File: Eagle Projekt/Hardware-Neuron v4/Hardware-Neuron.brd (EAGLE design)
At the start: 76.2 x 98.7 mm, 118 parts, among them Q1 FDN360P, Q10 BSS123, Q11 BSS123, Q12 BSS123, Q13 FDN360P, Q14 BCX71SMD, Q15 BCX71SMD, Q16 BSS123, Q17 BSS123, Q18 BSS123, Q19 BSS123, Q2 BCX71SMD, Q20 BSS123, Q21 BSS123, Q22 BCX71SMD, Q23 BCX71SMD, Q24 BSS123, Q25 BSS123, Q26 BSS123, Q27 BSS123, Q28 BSS123, Q29 BSS123, Q3 BCX71SMD, Q30 BSS123, Q31 BSS123, Q32 BSS123, Q33 BSS123, Q34 BSS123, Q35 BSS123, Q36 BSS123, Q37 BSS123, Q4 FDN360P, Q5 FDN360P, Q6 BSS123, Q7 BSS123, Q8 BSS123, Q9 FDN360P, T1 BC846, T2 BC846, T3 BC846, T4 BC846, T5 BC846, T6 BC846, T7 BC846, T8 BC846

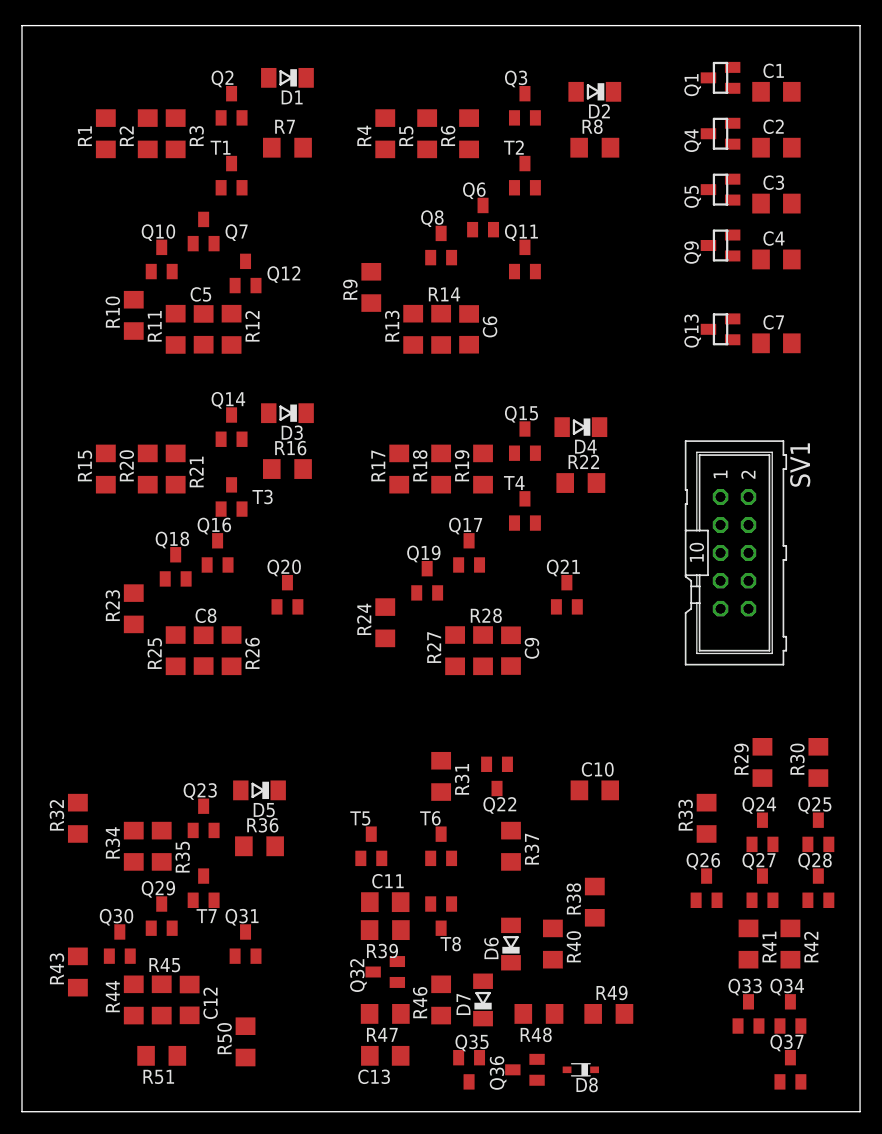
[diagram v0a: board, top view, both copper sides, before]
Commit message: Layout upgrade
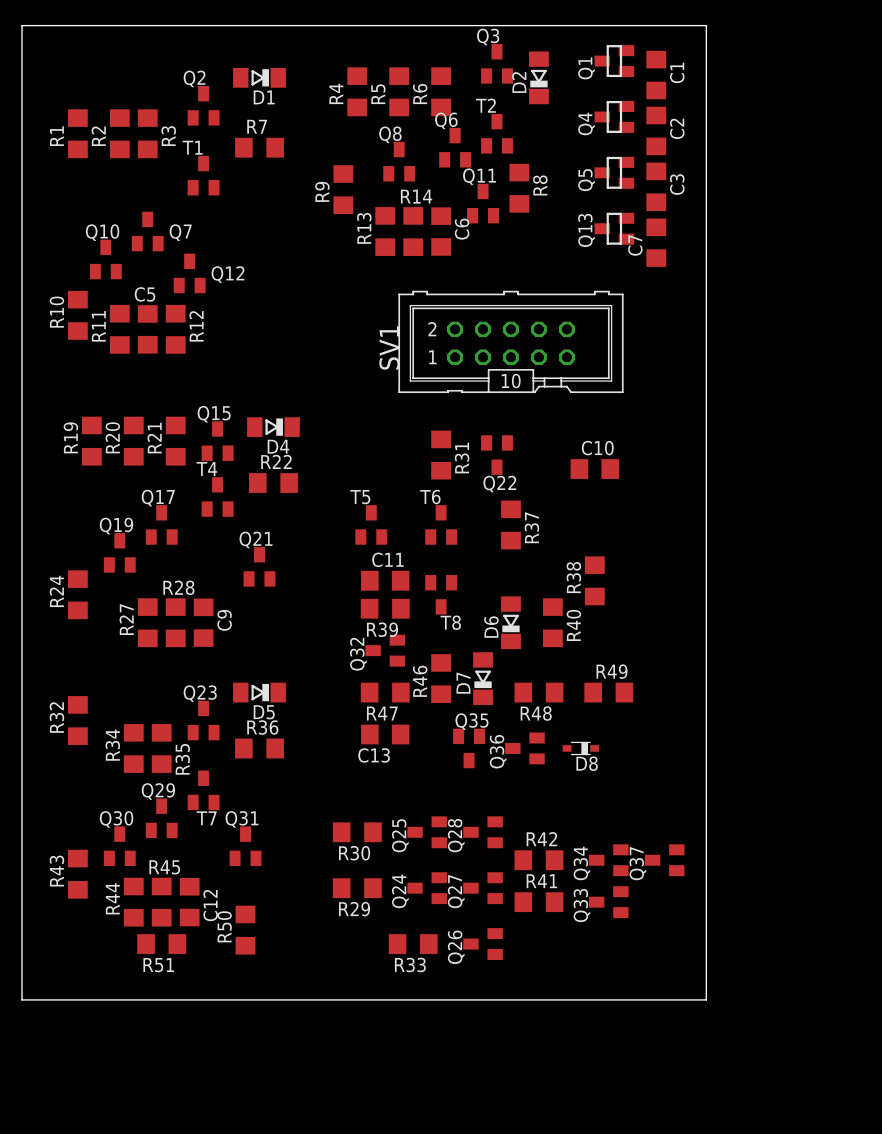
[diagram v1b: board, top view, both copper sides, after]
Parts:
- removed C4: 10n, rcl:C1206
- removed C8: 100n, rcl:C1206
- removed D3: PMLL41SOD80C, diode:SOD80C
- removed Q14: BCX71SMD, transistor-pnp:SOT23
- removed Q16, Q18, Q20: BSS123, transistor-small-signal:SOT23
- removed Q9: FDN360P, transistor-power:SUPER-SOT3
- removed R15, R17, R18, R23, R25, R26: 1kE, rcl:R1206
- removed R16: 10ME, rcl:R1206
- removed T3: BC846, transistor:SOT23
- moved R30 42.4 mm to (30.5, 25.4), turned to 180 degrees
- moved R29 38.6 mm to (30.5, 20.3), turned to 180 degrees
- moved R19 35.7 mm to (6.35, 61.0)
- moved Q25 35.6 mm to (36.8, 25.4), turned to 90 degrees
- moved Q24 30.9 mm to (36.8, 20.3), turned to 90 degrees
- moved Q28 30.9 mm to (41.9, 25.4), turned to 90 degrees
- moved D8 29.2 mm to (50.8, 33.0)
- moved Q35 29.2 mm to (40.6, 33.0)
- moved Q36 29.2 mm to (45.7, 33.0)
- moved R37 29.2 mm to (44.5, 53.3)
- moved T5 29.2 mm to (31.8, 53.3)
- moved T6 29.2 mm to (38.1, 53.3)
- moved C10 29.2 mm to (52.1, 58.4)
- moved C13 29.2 mm to (33.0, 34.3)
- moved D6 29.2 mm to (44.5, 44.5)
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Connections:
- removed net ENABLE: Q10.1, Q18.1, Q19.1, Q30.1, Q8.1, R10.2, R23.2, R24.2, R43.2, R9.2
- removed net N$44: Q16.3, R20.1, T3.1
- removed net N$45: Q14.2, R16.1, T3.3
- removed net N$46: D3.A, Q14.3
- removed net N$47: Q14.1, R15.2
- removed net N$48: Q16.1, Q18.3, R15.1, R21.1
- removed net N$49: Q18.2, Q20.3
- removed net OUT_3: C4.1, Q9.1, R16.2
- removed net X_3: C8.1, Q20.1, R25.2, R26.2
- net +5V: now also SV1.9; no longer R18.2, R19.2
- net 0V: now also SV1.10; no longer C4.2, C8.2, Q16.2, Q20.2, R23.1, R25.1, R26.1
- net A-Z: now also SV1.7; no longer Q9.3
- net DELTA: no longer D3.C, T3.2
- net EN: now also Q10.1, Q19.1, Q30.1, Q8.1, R10.2, R24.2, R43.2, R9.2, SV1.8
- net N$28: now also R21.1; no longer R19.1
- net N$39: now also R19.2; no longer R17.2
- net N$41: now also R19.1, R20.1; no longer R17.1, R18.1
- net X3: no longer Q9.2
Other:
- board size 76.2 x 98.7 mm -> 62.2 x 88.6 mm
